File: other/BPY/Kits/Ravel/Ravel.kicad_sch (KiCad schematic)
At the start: 5 parts, among them U1 ESP32-C3_SUPERMINI_TH

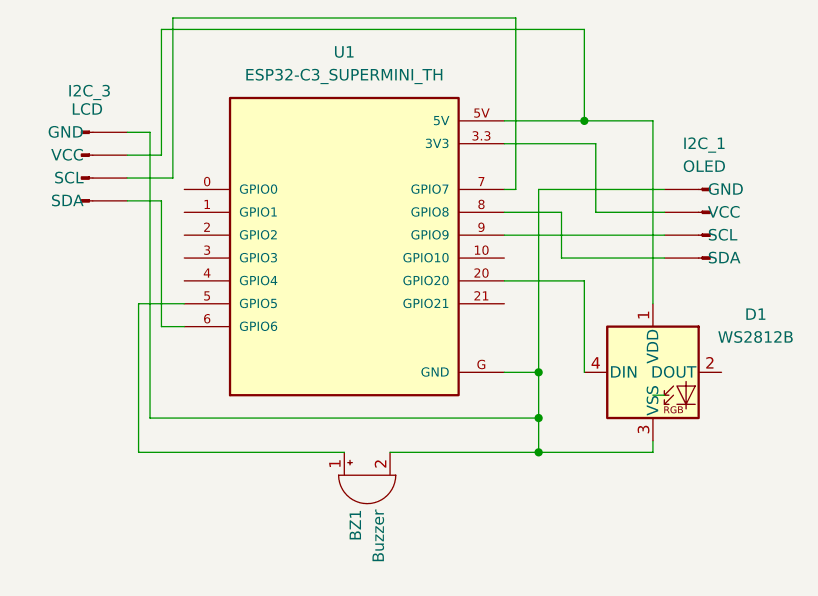
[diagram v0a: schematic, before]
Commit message: 22/02/2026 17:54:43
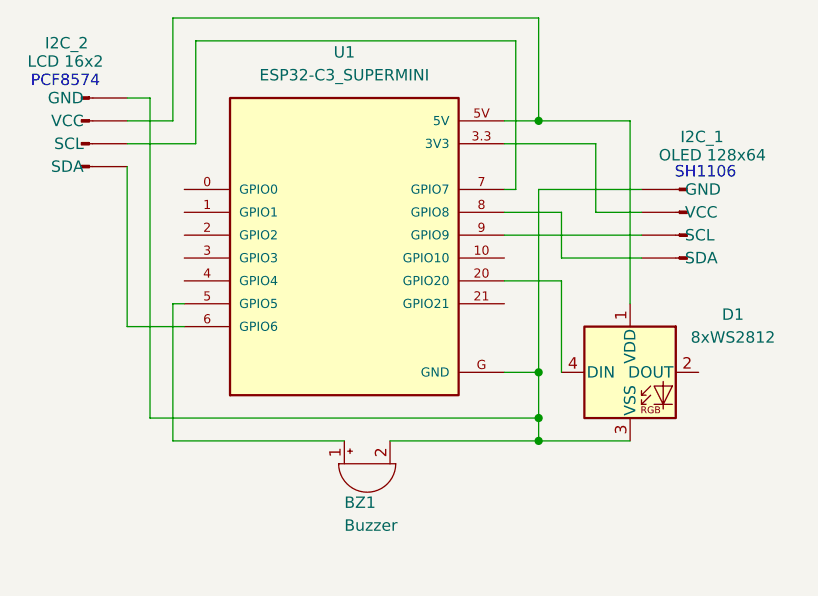
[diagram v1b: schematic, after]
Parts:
- D1: value WS2812B -> 8xWS2812
- I2C_1: value OLED -> OLED 128x64
- I2C_2: renamed from I2C_3; value LCD -> LCD 16x2
- U1: value ESP32-C3_SUPERMINI_TH -> ESP32-C3_SUPERMINI
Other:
- note added: "PCF8574"
- note added: "SH1106"
- company: (none) -> \nZelbinium\n(https://zelbinium.com)\n\n\n\n
- title: (none) -> Kit Ravel
- moved on the sheet: BZ1, D1, I2C_1, I2C_2
